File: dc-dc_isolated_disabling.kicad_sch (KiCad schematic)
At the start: 13 parts, among them Q201 2N7002, U201 CMP6793RE

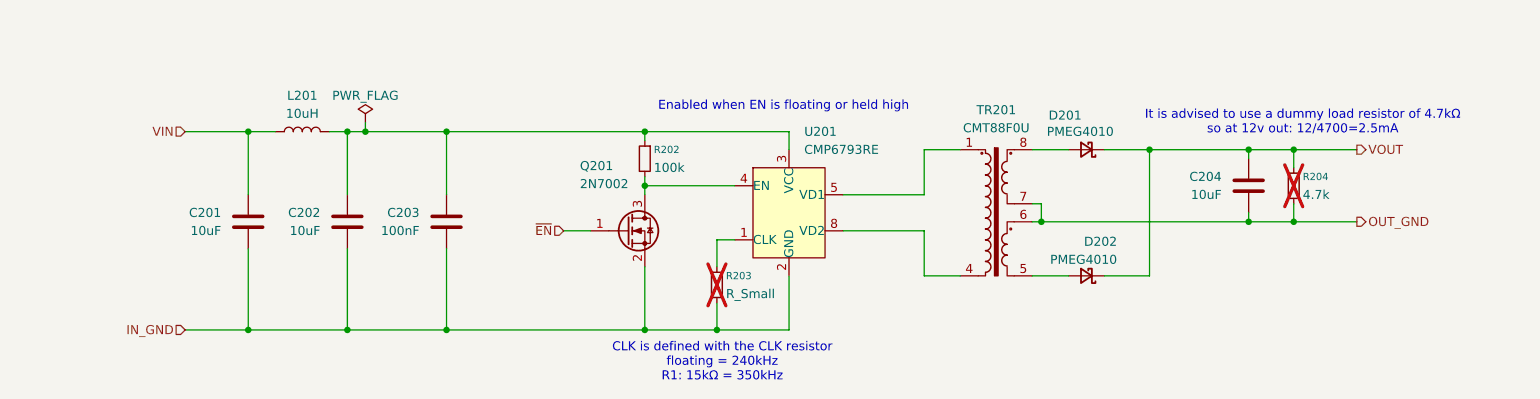
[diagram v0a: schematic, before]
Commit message: First layout complete - DRC not clear yet.
Signed-off-by: Jean Alinei <jean.alinei@owntech.org>
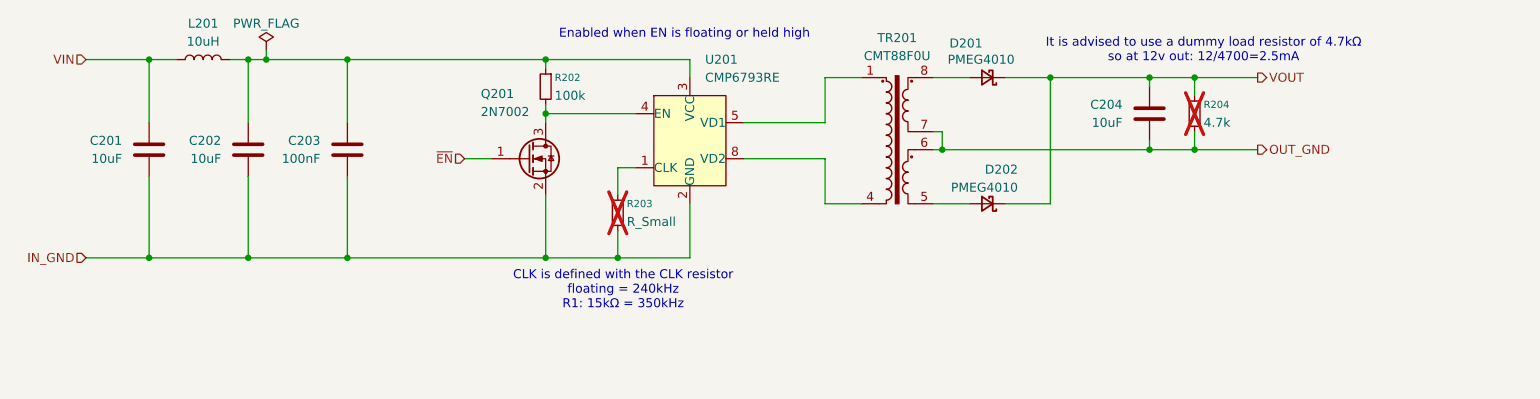
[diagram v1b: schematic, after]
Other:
- moved on the sheet: C201, C202, C203, C204, D201, D202, L201, Q201, R202, R203, R204, TR201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

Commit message: Found IC for ORing function. Added all LCSC refs. Found proper header stackup.
Signed-off-by: Jean Alinei <jean.alinei@owntech.org>
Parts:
- R202: LCSC (none) -> C15458
- TR201: LCSC (none) -> C37648313
